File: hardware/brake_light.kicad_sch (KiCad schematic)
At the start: 4 parts, among them Q5 PMV450ENEA

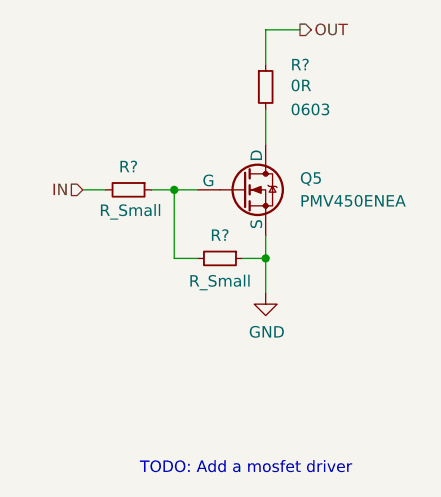
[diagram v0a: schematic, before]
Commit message: Add the Cube project
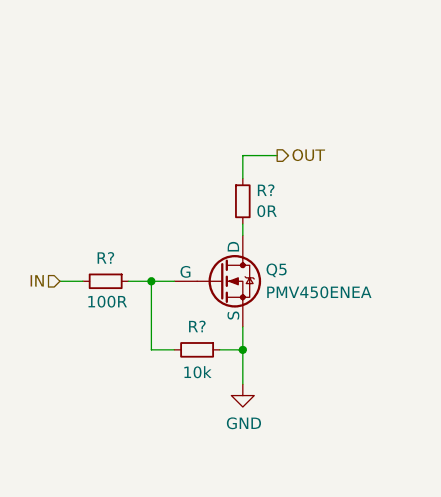
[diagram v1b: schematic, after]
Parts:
- R?: Case 0603 -> (none)
- R?: value R_Small -> 10k
- R?: value R_Small -> 100R
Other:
- note removed: "TODO: Add a mosfet driver"
- moved on the sheet: Q5, R?
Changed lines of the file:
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@@
   (paper "A4")
   (title_block
-    (date "2023-06-06")
+    (date "2023-07-01")
     (rev "${REVISION}")
     (company "Author: I. Kajdan")
     (comment 1 "Reviewer:")
   )
-  (junction (at 153.67 100.33) (diameter 0) (color 0 0 0 0)
+  (junction (at 151.13 110.49) (diameter 0) (color 0 0 0 0)
   )
-  (junction (at 143.51 92.71) (diameter 0) (color 0 0 0 0)
+  (junction (at 140.97 102.87) (diameter 0) (color 0 0 0 0)
   )
-  (wire (pts (xy 135.89 92.71) (xy 133.35 92.71))
+  (wire (pts (xy 133.35 102.87) (xy 130.81 102.87))
     (stroke (width 0) (type default))
   )
-  (wire (pts (xy 153.67 104.14) (xy 153.67 100.33))
+  (wire (pts (xy 151.13 114.3) (xy 151.13 110.49))
     (stroke (width 0) (type default))
   )
-  (wire (pts (xy 143.51 100.33) (xy 146.05 100.33))
+  (wire (pts (xy 140.97 110.49) (xy 143.51 110.49))
     (stroke (width 0) (type default))
   )
-  (wire (pts (xy 143.51 100.33) (xy 143.51 92.71))
+  (wire (pts (xy 140.97 110.49) (xy 140.97 102.87))
     (stroke (width 0) (type default))
   )
-  (wire (pts (xy 140.97 92.71) (xy 143.51 92.71))
+  (wire (pts (xy 138.43 102.87) (xy 140.97 102.87))
     (stroke (width 0) (type default))
   )
-  (wire (pts (xy 153.67 100.33) (xy 153.67 97.79))
+  (wire (pts (xy 151.13 110.49) (xy 151.13 107.95))
     (stroke (width 0) (type default))
   )
-  (wire (pts (xy 153.67 83.82) (xy 153.67 87.63))
+  (wire (pts (xy 151.13 96.52) (xy 151.13 97.79))
     (stroke (width 0) (type default))
   )
-  (wire (pts (xy 143.51 92.71) (xy 146.05 92.71))
+  (wire (pts (xy 140.97 102.87) (xy 143.51 102.87))
     (stroke (width 0) (type default))
   )
-  (wire (pts (xy 153.67 74.93) (xy 153.67 78.74))
+  (wire (pts (xy 151.13 88.9) (xy 151.13 91.44))
     (stroke (width 0) (type default))
   )
-  (wire (pts (xy 151.13 100.33) (xy 153.67 100.33))
+  (wire (pts (xy 148.59 110.49) (xy 151.13 110.49))
     (stroke (width 0) (type default))
   )
-  (wire (pts (xy 157.48 74.93) (xy 153.67 74.93))
+  (wire (pts (xy 154.94 88.9) (xy 151.13 88.9))
     (stroke (width 0) (type default))
   )
-  (text "TODO: Add a mosfet driver" (at 139.7 124.46 0)
-    (effects (font (size 1.27 1.27)) (justify left bottom))
-  )
-  (hierarchical_label "OUT" (shape output) (at 157.48 74.93 0) (fields_autoplaced)
+  (hierarchical_label "OUT" (shape output) (at 154.94 88.9 0) (fields_autoplaced)
     (effects (font (size 1.27 1.27)) (justify left))
   )
-  (hierarchical_label "IN" (shape input) (at 133.35 92.71 180) (fields_autoplaced)
+  (hierarchical_label "IN" (shape input) (at 130.81 102.87 180) (fields_autoplaced)
     (effects (font (size 1.27 1.27)) (justify right))
   )
-  (symbol (lib_id "Simulation_SPICE:NMOS") (at 151.13 92.71 0) (unit 1)
+  (symbol (lib_id "Simulation_SPICE:NMOS") (at 148.59 102.87 0) (unit 1)
     (in_bom yes) (on_board yes) (dnp no)
-    (property "Reference" "Q5" (at 157.48 91.44 0)
+    (property "Reference" "Q5" (at 153.67 101.6 0)
       (effects (font (size 1.27 1.27)) (justify left))
     )
-    (property "Value" "PMV450ENEA" (at 157.48 93.98 0)
+    (property "Value" "PMV450ENEA" (at 153.67 104.14 0)
       (effects (font (size 1.27 1.27)) (justify left))
     )
-    (property "Footprint" "" (at 156.21 90.17 0)
+    (property "Footprint" "" (at 153.67 100.33 0)
       (effects (font (size 1.27 1.27)) hide)
     )
-    (property "Datasheet" "https://assets.nexperia.com/documents/data-sheet/PMV450ENEA.pdf" (at 151.13 105.41 0)
+    (property "Datasheet" "https://assets.nexperia.com/documents/data-sheet/PMV450ENEA.pdf" (at 148.59 115.57 0)
       (effects (font (size 1.27 1.27)) hide)
     )
@@
     )
   )
-  (symbol (lib_id "Device:R_Small") (at 153.67 81.28 0) (unit 1)
+  (symbol (lib_id "Device:R_Small") (at 151.13 93.98 0) (unit 1)
     (in_bom yes) (on_board yes) (dnp no)
-    (property "Reference" "R?" (at 156.4386 78.8416 0)
+    (property "Reference" "R?" (at 152.6286 92.8116 0)
       (effects (font (size 1.27 1.27)) (justify left))
     )
-    (property "Value" "0R" (at 156.4386 81.153 0)
+    (property "Value" "0R" (at 152.6286 95.123 0)
       (effects (font (size 1.27 1.27)) (justify left))
     )
-    (property "Footprint" "Resistor_SMD:R_0603_1608Metric" (at 153.67 81.28 0)
+    (property "Footprint" "Resistor_SMD:R_0603_1608Metric" (at 151.13 93.98 0)
       (effects (font (size 1.27 1.27)) hide)
     )
-    (property "Datasheet" "~" (at 153.67 81.28 0)
+    (property "Datasheet" "~" (at 151.13 93.98 0)
       (effects (font (size 1.27 1.27)) hide)
-    )
-    (property "Case" "0603" (at 156.4386 83.82 0)
-      (effects (font (size 1.27 1.27)) (justify left))
     )
     (pin "1")
@@
     )
   )
-  (symbol (lib_id "Device:R_Small") (at 148.59 100.33 270) (unit 1)
+  (symbol (lib_id "Device:R_Small") (at 146.05 110.49 270) (unit 1)
     (in_bom yes) (on_board yes) (dnp no)
-    (property "Reference" "R?" (at 148.59 97.79 90)
+    (property "Reference" "R?" (at 146.05 107.95 90)
       (effects (font (size 1.27 1.27)))
     )
-    (property "Value" "R_Small" (at 148.59 102.87 90)
+    (property "Value" "10k" (at 146.05 113.03 90)
       (effects (font (size 1.27 1.27)))
     )
-    (property "Footprint" "Resistor_SMD:R_0402_1005Metric" (at 148.59 100.33 0)
+    (property "Footprint" "Resistor_SMD:R_0402_1005Metric" (at 146.05 110.49 0)
       (effects (font (size 1.27 1.27)) hide)
     )
-    (property "Datasheet" "~" (at 148.59 100.33 0)
+    (property "Datasheet" "~" (at 146.05 110.49 0)
       (effects (font (size 1.27 1.27)) hide)
     )
@@
     )
   )
-  (symbol (lib_id "power:GND") (at 153.67 104.14 0) (unit 1)
+  (symbol (lib_id "power:GND") (at 151.13 114.3 0) (unit 1)
     (in_bom yes) (on_board yes) (dnp no)
-    (property "Reference" "#PWR?" (at 153.67 110.49 0)
+    (property "Reference" "#PWR?" (at 151.13 120.65 0)
       (effects (font (size 1.27 1.27)) hide)
     )
-    (property "Value" "GND" (at 153.797 108.5342 0)
+    (property "Value" "GND" (at 151.257 118.6942 0)
       (effects (font (size 1.27 1.27)))
     )
-    (property "Footprint" "" (at 153.67 104.14 0)
+    (property "Footprint" "" (at 151.13 114.3 0)
       (effects (font (size 1.27 1.27)) hide)
     )
-    (property "Datasheet" "" (at 153.67 104.14 0)
+    (property "Datasheet" "" (at 151.13 114.3 0)
       (effects (font (size 1.27 1.27)) hide)
     )
@@
     )
   )
-  (symbol (lib_id "Device:R_Small") (at 138.43 92.71 270) (unit 1)
+  (symbol (lib_id "Device:R_Small") (at 135.89 102.87 270) (unit 1)
     (in_bom yes) (on_board yes) (dnp no)
-    (property "Reference" "R?" (at 138.43 90.17 90)
+    (property "Reference" "R?" (at 135.89 100.33 90)
       (effects (font (size 1.27 1.27)))
     )
-    (property "Value" "R_Small" (at 142.113 95.0214 90)
+    (property "Value" "100R" (at 138.303 105.1814 90)
       (effects (font (size 1.27 1.27)) (justify right))
     )
-    (property "Footprint" "Resistor_SMD:R_0402_1005Metric" (at 138.43 92.71 0)
+    (property "Footprint" "Resistor_SMD:R_0402_1005Metric" (at 135.89 102.87 0)
       (effects (font (size 1.27 1.27)) hide)
     )
-    (property "Datasheet" "~" (at 138.43 92.71 0)
+    (property "Datasheet" "~" (at 135.89 102.87 0)
       (effects (font (size 1.27 1.27)) hide)
     )
